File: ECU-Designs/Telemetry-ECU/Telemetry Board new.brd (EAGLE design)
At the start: 37.5 x 45.7 mm, 9 parts, among them X1 Suspension Sensor, X2 Wheel Sensor, X3 Tire Temperature Sensor, X5 MINIFIT_5566-4

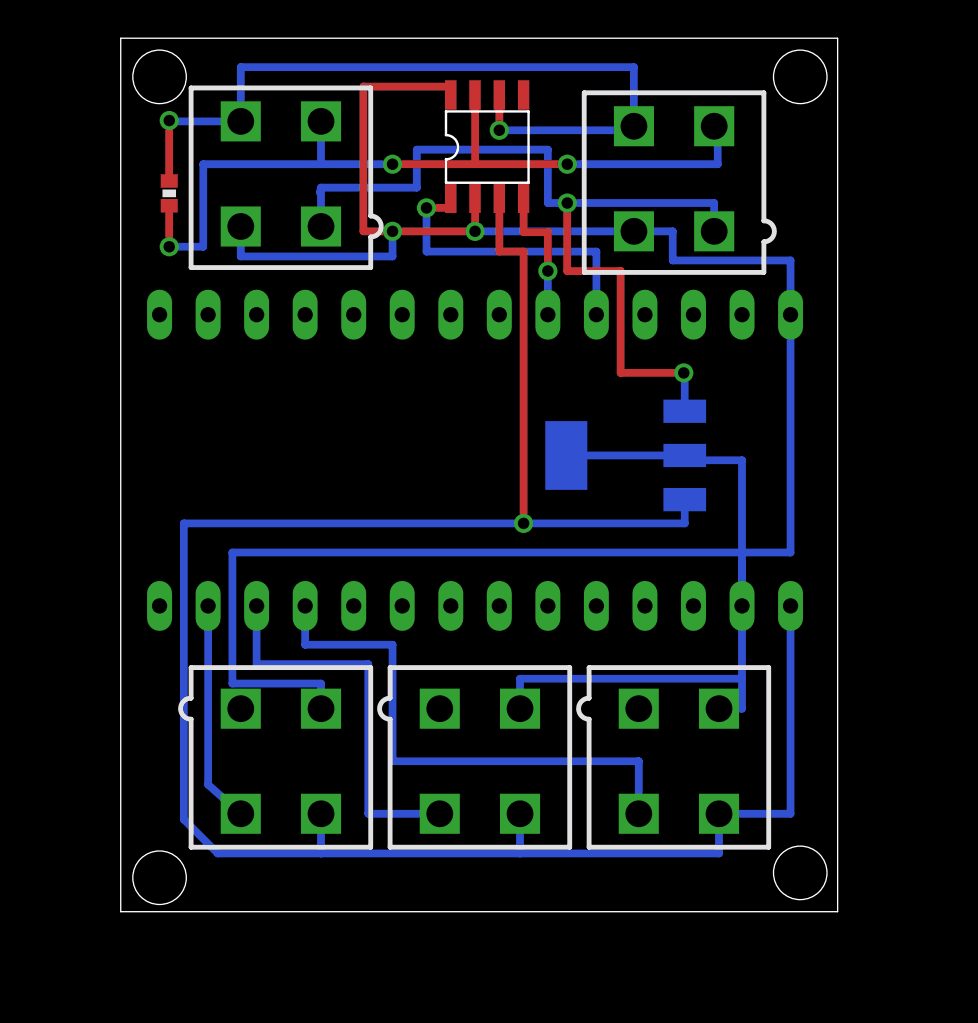
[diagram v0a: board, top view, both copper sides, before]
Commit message: Hopefully the final working of the Telemetry BRD
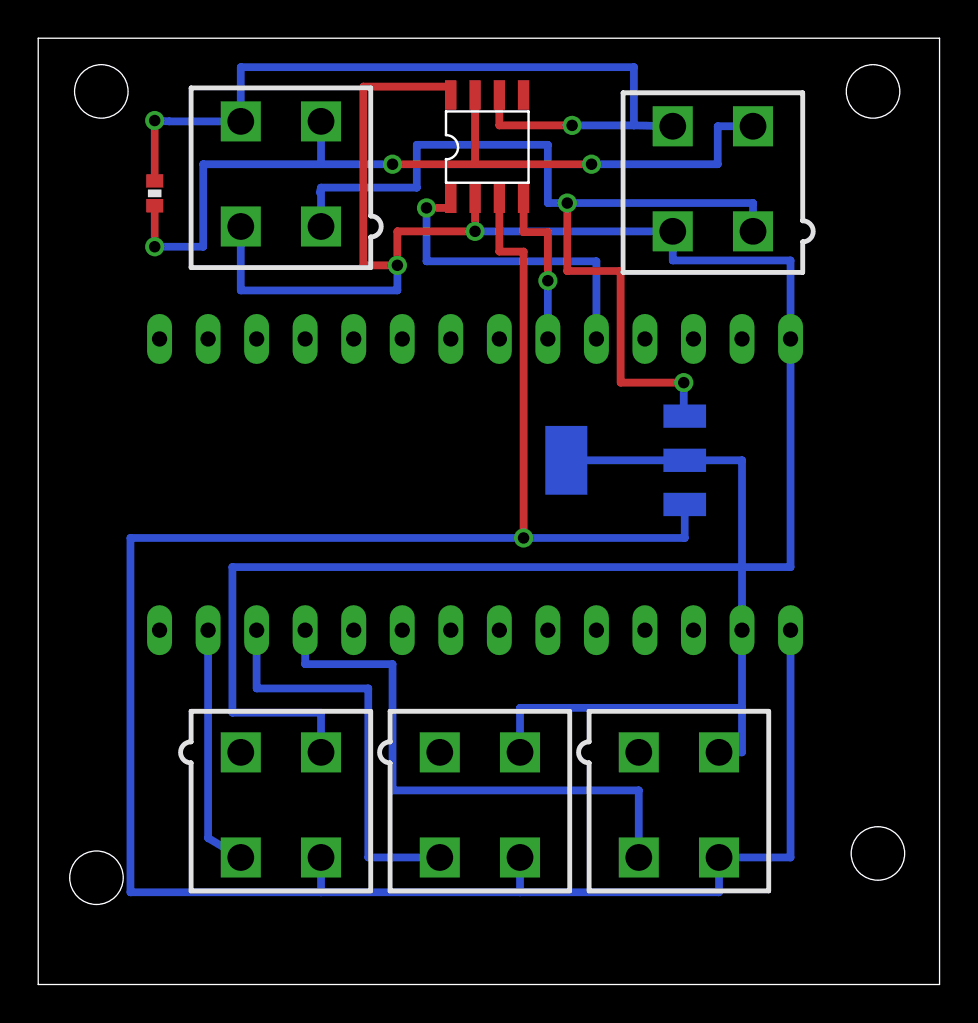
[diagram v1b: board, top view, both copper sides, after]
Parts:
- moved X1 2.29 mm to (58.4, 11.7)
- moved X2 2.29 mm to (37.6, 11.7)
- moved X3 2.29 mm to (48.0, 11.7)
- moved X5 2.03 mm to (60.2, 44.5)
- moved U$1 1.27 mm to (30.0, 37.3)
- moved 120 0.76 mm to (31.0, 43.7)
- moved U$3 0.25 mm to (55.6, 29.7)
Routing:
- net N$13: track 110.8 -> 120.3 mm
- net N$6: track 145.4 -> 153.8 mm
- net N$1: track 46.2 -> 49.0 mm
- net N$3: track 43.2 -> 45.6 mm
- net N$4: track 42.5 -> 44.8 mm
- net N$9: track 16.3 -> 17.5 mm
- net N$10: track 7.37 -> 8.64 mm
- net N$16: track 11.6 -> 12.9 mm
- net N$12: track 20.5 -> 21.5 mm
- net N$19: track 28.3 -> 29.4 mm
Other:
- board size 37.5 x 45.7 mm -> 47.2 x 49.5 mm
